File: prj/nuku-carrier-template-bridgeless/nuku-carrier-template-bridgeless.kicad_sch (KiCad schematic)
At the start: 0 parts

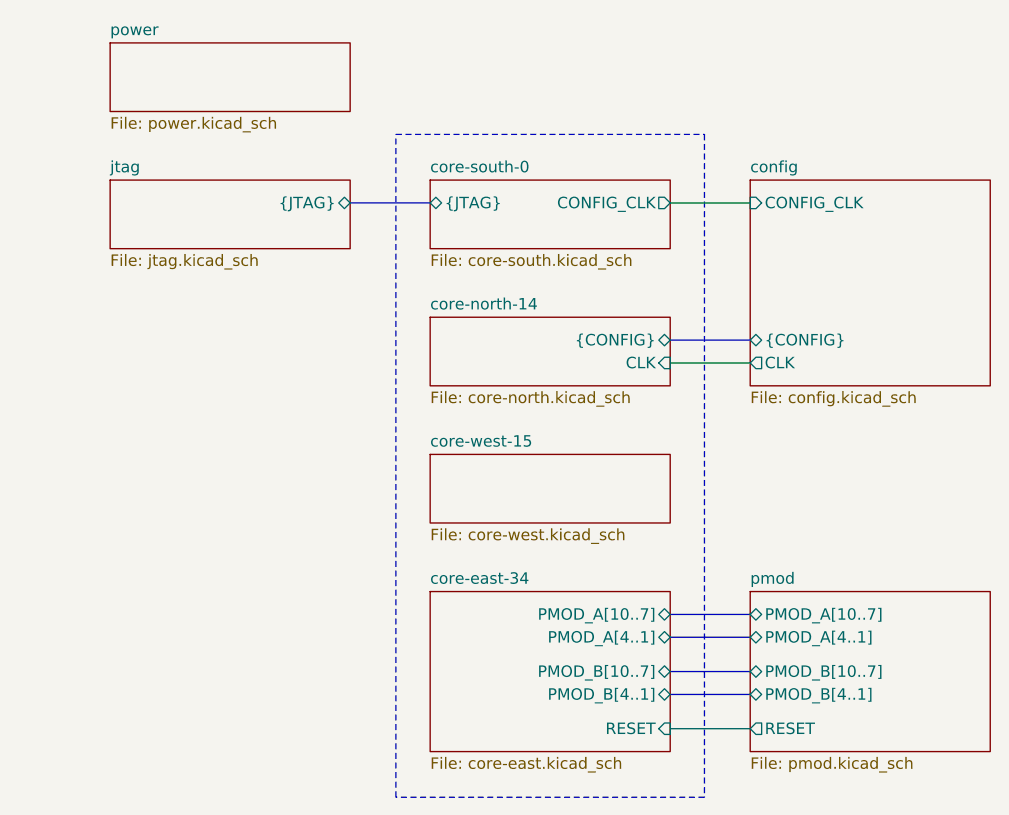
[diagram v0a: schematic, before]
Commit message: Finish boards - prod ready
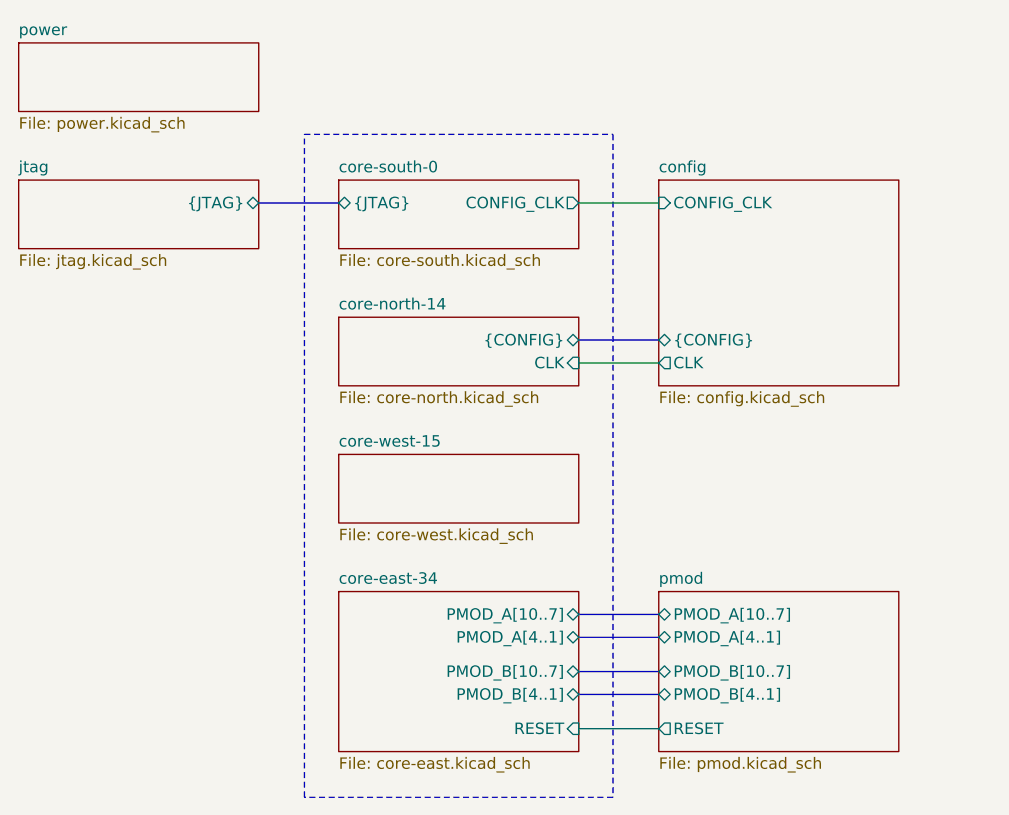
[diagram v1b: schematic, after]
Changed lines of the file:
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@@
 	)
 	(rectangle
-		(start 138.43 66.04)
-		(end 172.72 139.7)
+		(start 128.27 66.04)
+		(end 162.56 139.7)
 		(stroke
 			(width 0)
@@
 	(bus
 		(pts
-			(xy 168.91 121.92) (xy 177.8 121.92)
+			(xy 158.75 121.92) (xy 167.64 121.92)
 		)
 		(stroke
@@
 	(bus
 		(pts
-			(xy 168.91 125.73) (xy 177.8 125.73)
+			(xy 158.75 125.73) (xy 167.64 125.73)
 		)
 		(stroke
@@
 	(bus
 		(pts
-			(xy 168.91 119.38) (xy 177.8 119.38)
+			(xy 158.75 119.38) (xy 167.64 119.38)
 		)
 		(stroke
@@
 	(bus
 		(pts
-			(xy 168.91 88.9) (xy 177.8 88.9)
+			(xy 158.75 88.9) (xy 167.64 88.9)
 		)
 		(stroke
@@
 	(bus
 		(pts
-			(xy 133.35 73.66) (xy 142.24 73.66)
+			(xy 123.19 73.66) (xy 132.08 73.66)
 		)
 		(stroke
@@
 	(wire
 		(pts
-			(xy 168.91 73.66) (xy 177.8 73.66)
+			(xy 158.75 73.66) (xy 167.64 73.66)
 		)
 		(stroke
@@
 	(bus
 		(pts
-			(xy 168.91 128.27) (xy 177.8 128.27)
+			(xy 158.75 128.27) (xy 167.64 128.27)
 		)
 		(stroke
@@
 	(wire
 		(pts
-			(xy 168.91 91.44) (xy 177.8 91.44)
+			(xy 158.75 91.44) (xy 167.64 91.44)
 		)
 		(stroke
@@
 	(wire
 		(pts
-			(xy 168.91 132.08) (xy 177.8 132.08)
-		)
-		(stroke
-			(width 0)
-			(type default)
-		)
-	)
-	(sheet
-		(at 106.68 55.88)
+			(xy 158.75 132.08) (xy 167.64 132.08)
+		)
+		(stroke
+			(width 0)
+			(type default)
+		)
+	)
+	(sheet
+		(at 96.52 55.88)
 		(size 26.67 7.62)
 		(exclude_from_sim no)
@@
 		)
 		(property "Sheetname" "power"
-			(at 106.68 55.1684 0)
+			(at 96.52 55.1684 0)
 			(effects
 				(font
@@
 		)
 		(property "Sheetfile" "power.kicad_sch"
-			(at 106.68 64.0846 0)
+			(at 96.52 64.0846 0)
 			(effects
 				(font
@@
 	)
 	(sheet
-		(at 142.24 86.36)
+		(at 132.08 86.36)
 		(size 26.67 7.62)
 		(exclude_from_sim no)
@@
 		)
 		(property "Sheetname" "core-north-14"
-			(at 142.24 85.6484 0)
+			(at 132.08 85.6484 0)
 			(effects
 				(font
@@
 		)
 		(property "Sheetfile" "core-north.kicad_sch"
-			(at 142.24 94.5646 0)
+			(at 132.08 94.5646 0)
 			(effects
 				(font
@@
 		)
 		(pin "CLK" input
-			(at 168.91 91.44 0)
+			(at 158.75 91.44 0)
 			(effects
 				(font
@@
 		)
 		(pin "{CONFIG}" bidirectional
-			(at 168.91 88.9 0)
+			(at 158.75 88.9 0)
 			(effects
 				(font
@@
 	)
 	(sheet
-		(at 177.8 71.12)
+		(at 167.64 71.12)
 		(size 26.67 22.86)
 		(exclude_from_sim no)
@@
 		)
 		(property "Sheetname" "config"
-			(at 177.8 70.4084 0)
+			(at 167.64 70.4084 0)
 			(effects
 				(font
@@
 		)
 		(property "Sheetfile" "config.kicad_sch"
-			(at 177.8 94.5646 0)
+			(at 167.64 94.5646 0)
 			(effects
 				(font
@@
 		)
 		(pin "CLK" output
-			(at 177.8 91.44 180)
+			(at 167.64 91.44 180)
 			(effects
 				(font
@@
 		)
 		(pin "CONFIG_CLK" input
-			(at 177.8 73.66 180)
+			(at 167.64 73.66 180)
 			(effects
 				(font
@@
 		)
 		(pin "{CONFIG}" bidirectional
-			(at 177.8 88.9 180)
+			(at 167.64 88.9 180)
 			(effects
 				(font
@@
 	)
 	(sheet
-		(at 106.68 71.12)
+		(at 96.52 71.12)
 		(size 26.67 7.62)
 		(exclude_from_sim no)
@@
 		)
 		(property "Sheetname" "jtag"
-			(at 106.68 70.4084 0)
+			(at 96.52 70.4084 0)
 			(effects
 				(font
@@
 		)
 		(property "Sheetfile" "jtag.kicad_sch"
-			(at 106.68 79.3246 0)
+			(at 96.52 79.3246 0)
 			(effects
 				(font
@@
 		)
 		(pin "{JTAG}" bidirectional
-			(at 133.35 73.66 0)
+			(at 123.19 73.66 0)
 			(effects
 				(font
@@
 	)
 	(sheet
-		(at 142.24 116.84)
+		(at 132.08 116.84)
 		(size 26.67 17.78)
 		(exclude_from_sim no)
@@
 		)
 		(property "Sheetname" "core-east-34"
-			(at 142.24 116.1284 0)
+			(at 132.08 116.1284 0)
 			(effects
 				(font
@@
 		)
 		(property "Sheetfile" "core-east.kicad_sch"
-			(at 142.24 135.2046 0)
+			(at 132.08 135.2046 0)
 			(effects
 				(font
@@
 		)
 		(pin "PMOD_A[4..1]" bidirectional
-			(at 168.91 121.92 0)
+			(at 158.75 121.92 0)
 			(effects
 				(font
@@
 		)
 		(pin "PMOD_A[10..7]" bidirectional
-			(at 168.91 119.38 0)
+			(at 158.75 119.38 0)
 			(effects
 				(font
@@
 		)
 		(pin "PMOD_B[4..1]" bidirectional
-			(at 168.91 128.27 0)
+			(at 158.75 128.27 0)
 			(effects
 				(font
@@
 		)
 		(pin "PMOD_B[10..7]" bidirectional
-			(at 168.91 125.73 0)
+			(at 158.75 125.73 0)
 			(effects
 				(font
@@
 		)
 		(pin "RESET" input
-			(at 168.91 132.08 0)
+			(at 158.75 132.08 0)
 			(effects
 				(font
@@
 	)
 	(sheet
-		(at 177.8 116.84)
+		(at 167.64 116.84)
 		(size 26.67 17.78)
 		(exclude_from_sim no)
@@
 		)
 		(property "Sheetname" "pmod"
-			(at 177.8 116.1284 0)
+			(at 167.64 116.1284 0)
 			(effects
 				(font
@@
 		)
 		(property "Sheetfile" "pmod.kicad_sch"
-			(at 177.8 135.2046 0)
+			(at 167.64 135.2046 0)
 			(effects
 				(font
@@
 		)
 		(pin "PMOD_A[4..1]" bidirectional
-			(at 177.8 121.92 180)
+			(at 167.64 121.92 180)
 			(effects
 				(font
@@
 		)
 		(pin "PMOD_A[10..7]" bidirectional
-			(at 177.8 119.38 180)
+			(at 167.64 119.38 180)
 			(effects
 				(font
@@
 		)
 		(pin "PMOD_B[4..1]" bidirectional
-			(at 177.8 128.27 180)
+			(at 167.64 128.27 180)
 			(effects
 				(font
@@
 		)
 		(pin "PMOD_B[10..7]" bidirectional
-			(at 177.8 125.73 180)
+			(at 167.64 125.73 180)
 			(effects
 				(font
@@
 		)
 		(pin "RESET" output
-			(at 177.8 132.08 180)
+			(at 167.64 132.08 180)
 			(effects
 				(font
@@
 	)
 	(sheet
-		(at 142.24 71.12)
+		(at 132.08 71.12)
 		(size 26.67 7.62)
 		(exclude_from_sim no)
@@
 		)
 		(property "Sheetname" "core-south-0"
-			(at 142.24 70.4084 0)
+			(at 132.08 70.4084 0)
 			(effects
 				(font
@@
 		)
 		(property "Sheetfile" "core-south.kicad_sch"
-			(at 142.24 79.3246 0)
+			(at 132.08 79.3246 0)
 			(effects
 				(font
@@
 		)
 		(pin "CONFIG_CLK" output
-			(at 168.91 73.66 0)
+			(at 158.75 73.66 0)
 			(effects
 				(font
@@
 		)
 		(pin "{JTAG}" bidirectional
-			(at 142.24 73.66 180)
+			(at 132.08 73.66 180)
 			(effects
 				(font
@@
 	)
 	(sheet
-		(at 142.24 101.6)
+		(at 132.08 101.6)
 		(size 26.67 7.62)
 		(exclude_from_sim no)
@@
 		)
 		(property "Sheetname" "core-west-15"
-			(at 142.24 100.8884 0)
+			(at 132.08 100.8884 0)
 			(effects
 				(font
@@
 		)
 		(property "Sheetfile" "core-west.kicad_sch"
-			(at 142.24 109.8046 0)
-			(effects
-				(font
+			(at 132.08 109.8046 0)
+			(effects
+				(font
